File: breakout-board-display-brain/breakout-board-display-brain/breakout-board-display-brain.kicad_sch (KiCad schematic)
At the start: 7 parts, among them J1 Conn_01x19_Socket, J2 Conn_01x19_Socket, J3 Conn_01x16_Female, J4 Conn_01x16_Socket, J5 Conn_01x11_Socket, SW1 RotaryEncoder_Switch, U1 ESP32-WROOM-32

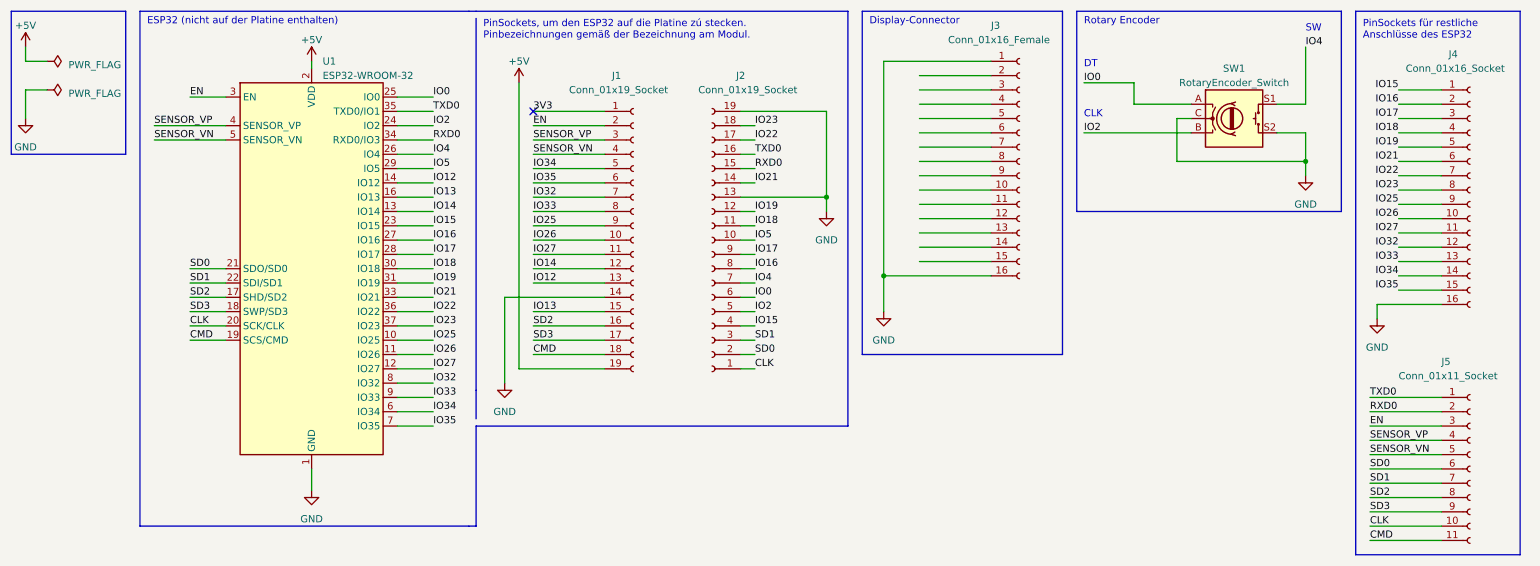
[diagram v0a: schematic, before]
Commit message: finsihed breakout-board.display-brain
fertig fürs Fräsen
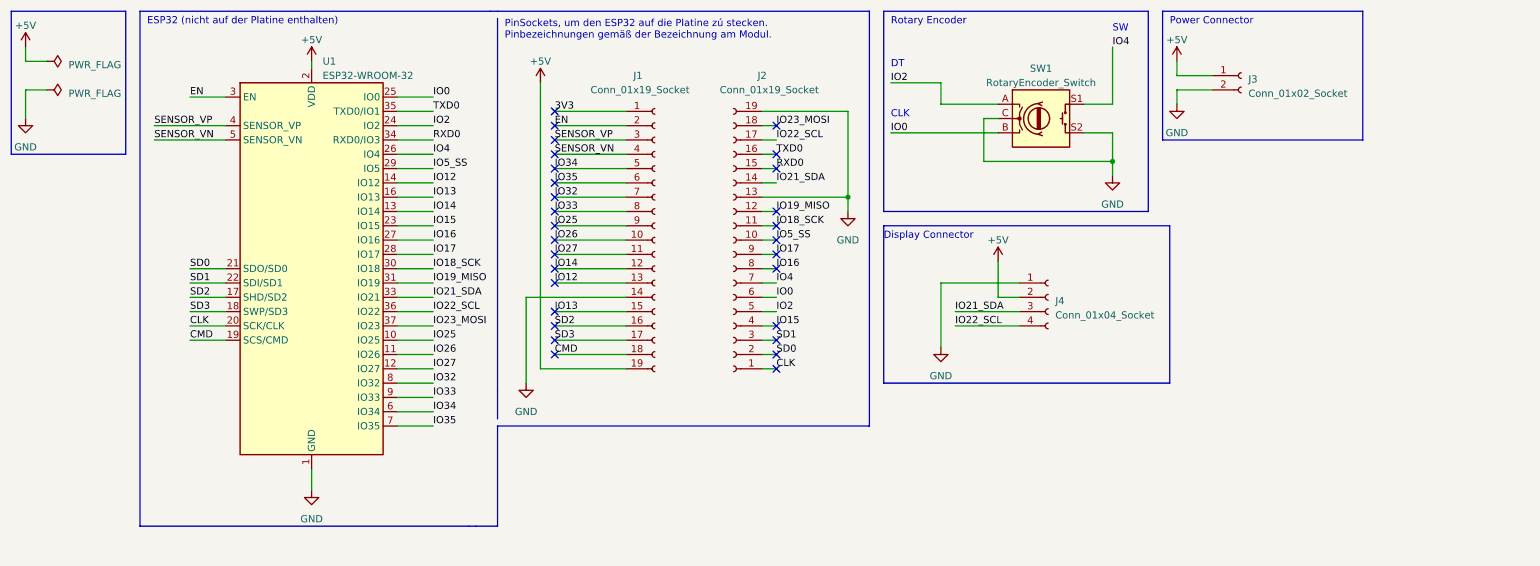
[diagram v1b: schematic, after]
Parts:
- removed J3: Conn_01x16_Female, Connector_PinSocket_2.54mm:PinSocket_1x16_P2.54mm_Vertical, symbol Connector:Conn_01x16_Female
- removed J4: Conn_01x16_Socket, symbol Connector:Conn_01x16_Socket
- removed J5: Conn_01x11_Socket, symbol Connector:Conn_01x11_Socket
- added J3: Conn_01x02_Socket, Connector_PinSocket_2.54mm:PinSocket_1x02_P2.54mm_Vertical, symbol Connector:Conn_01x02_Socket
- added J4: Conn_01x04_Socket, Connector_PinSocket_2.54mm:PinSocket_1x04_P2.54mm_Vertical, symbol Connector:Conn_01x04_Socket
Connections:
- net +5V: now also J3.1 (Pin_1), J4.2 (Pin_2)
- net GND: now also J3.2 (Pin_2), J4.1 (Pin_1)
- net IO0: now also SW1.B; no longer SW1.A
- net IO2: now also SW1.A; no longer SW1.B
- net IO18 renamed IO18_SCK
- net IO19 renamed IO19_MISO
- net IO21 renamed IO21_SDA
- net IO21_SDA: now also J4.3 (Pin_3)
- net IO22 renamed IO22_SCL
- net IO22_SCL: now also J4.4 (Pin_4)
- net IO23 renamed IO23_MOSI
- net IO5 renamed IO5_SS
- no-connect marks 1 -> 29
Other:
- note added: "Display Connector"
- note added: "Power Connector"
- note removed: "Display-Connector"
- note removed: "PinSockets für restliche Anschlüsse des ESP32"
- moved on the sheet: J1, J2, SW1
